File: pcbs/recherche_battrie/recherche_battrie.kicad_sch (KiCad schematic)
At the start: 5 parts, among them Q1 Q_Dual_NMOS_S1G1D2S2G2D1, U1 TP4056-42-ESOP8, U2 DW01A, U3 ME6211C33M5, U4 TPL5110

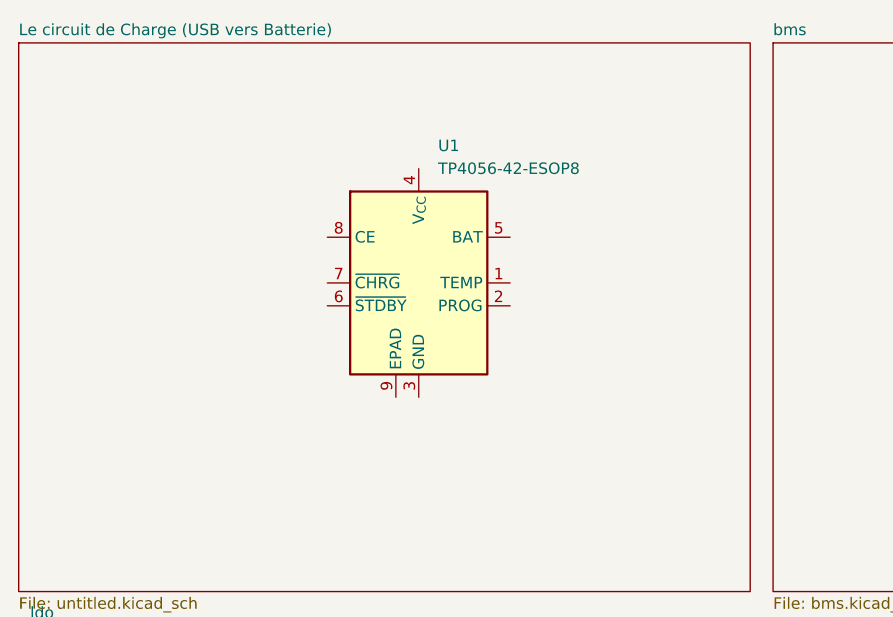
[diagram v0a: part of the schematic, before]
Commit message: mise a jour
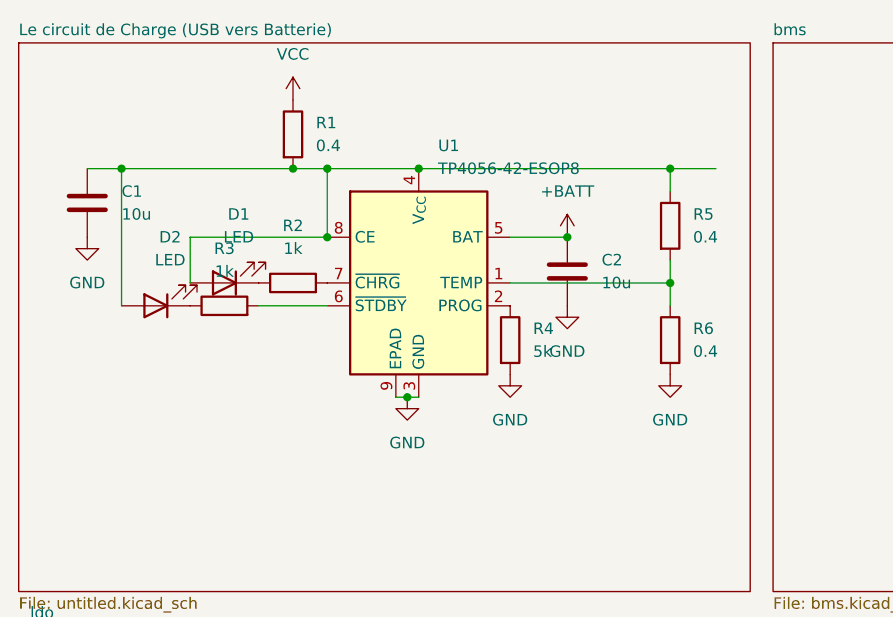
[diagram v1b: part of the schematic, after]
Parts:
- added C1, C2: 10u, symbol Device:C
- added D1, D2: LED, symbol Device:LED
- added R1, R5, R6: 0.4, symbol Device:R
- added R2, R3: 1k, symbol Device:R
- added R4: 5k, symbol Device:R
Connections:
- net at U1.1 (TEMP): now also R5.2, R6.1
- net at U1.2 (PROG): now also R4.1
- net GND: now reaches U1.3 (GND)
- net GND: now also U1.9 (EPAD), C1.2, C2.2, R4.2, R6.2
- net at U1.4 (V_{CC}): now also U1.8 (CE), C1.1, D1.2 (A), D2.2 (A), R1.2, R5.1
- net +BATT: now reaches U1.5 (BAT)
- net +BATT: now also C2.1
- net at U1.6 (~{STDBY}): now also R3.2
- net at U1.7 (~{CHRG}): now also R2.2
- new net: D1.1 (K), R2.1
- new net: D2.1 (K), R3.1
- new net VCC: R1.1
